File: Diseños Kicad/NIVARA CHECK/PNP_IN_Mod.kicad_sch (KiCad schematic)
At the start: 3 parts, among them U5 LTV-357T

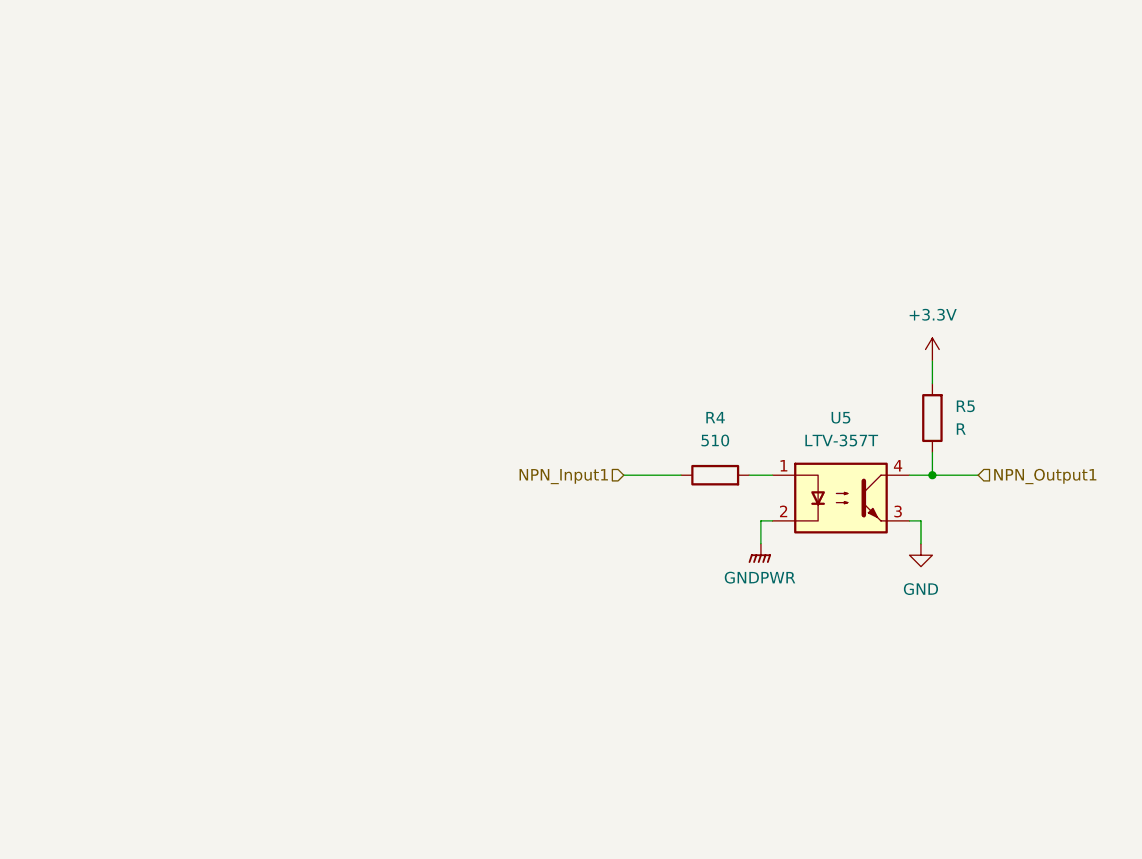
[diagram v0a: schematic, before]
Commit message: ACTUALIZACION HECHA
PCB SUPUESTA
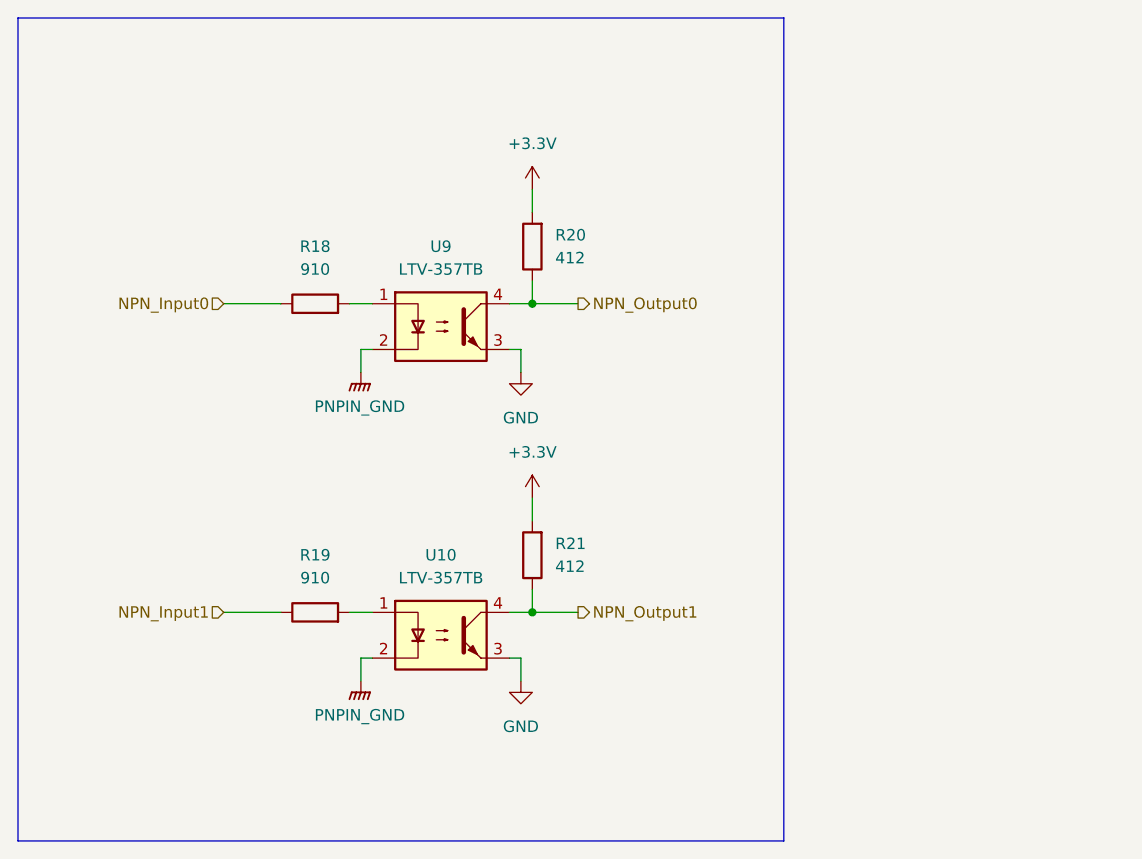
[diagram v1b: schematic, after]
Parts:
- removed R4: 510, Resistor_SMD:R_0603_1608Metric, symbol Device:R
- removed R5: R, symbol Device:R
- removed U5: LTV-357T, Package_SO:SO-4_4.4x3.6mm_P2.54mm, symbol Isolator:LTV-357T
- added R18, R19: 910, Resistor_SMD:R_0603_1608Metric, symbol Device:R
- added R20, R21: 412, symbol Device:R
- added U10, U9: LTV-357TB, Package_SO:SO-4_4.4x3.6mm_P2.54mm, symbol Isolator:LTV-357T
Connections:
- net +3.3V: now also R20.2, R21.2
- net GND: now also U10.3, U9.3
- net NPN_Input1: now also R19.1
- net NPN_Output1: now also R21.1, U10.4
- new net: R19.2, U10.1
- new net: R18.2, U9.1
- new net NPN_Input0: R18.1
- new net NPN_Output0: R20.1, U9.4
- new net PNPIN_GND: U10.2, U9.2
